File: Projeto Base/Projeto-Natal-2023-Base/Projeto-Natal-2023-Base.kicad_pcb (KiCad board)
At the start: 2 copper layers, 50 x 50 mm, 54 parts, among them J1 Conn_01x03_Pin, Q1 BC817, Q2 BC817, Q3 BC817, Q4 BC817, U1 CH32V003F4P6

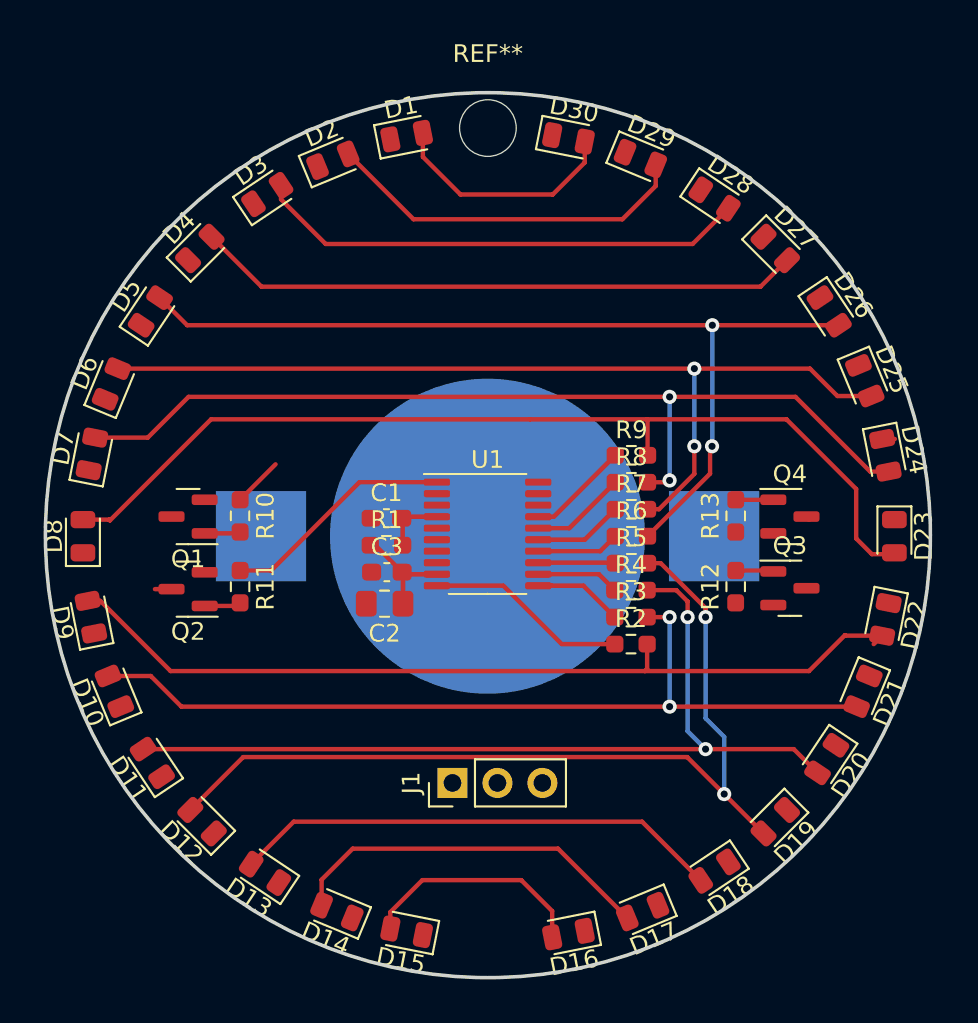
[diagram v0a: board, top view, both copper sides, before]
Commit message: v1.0.0
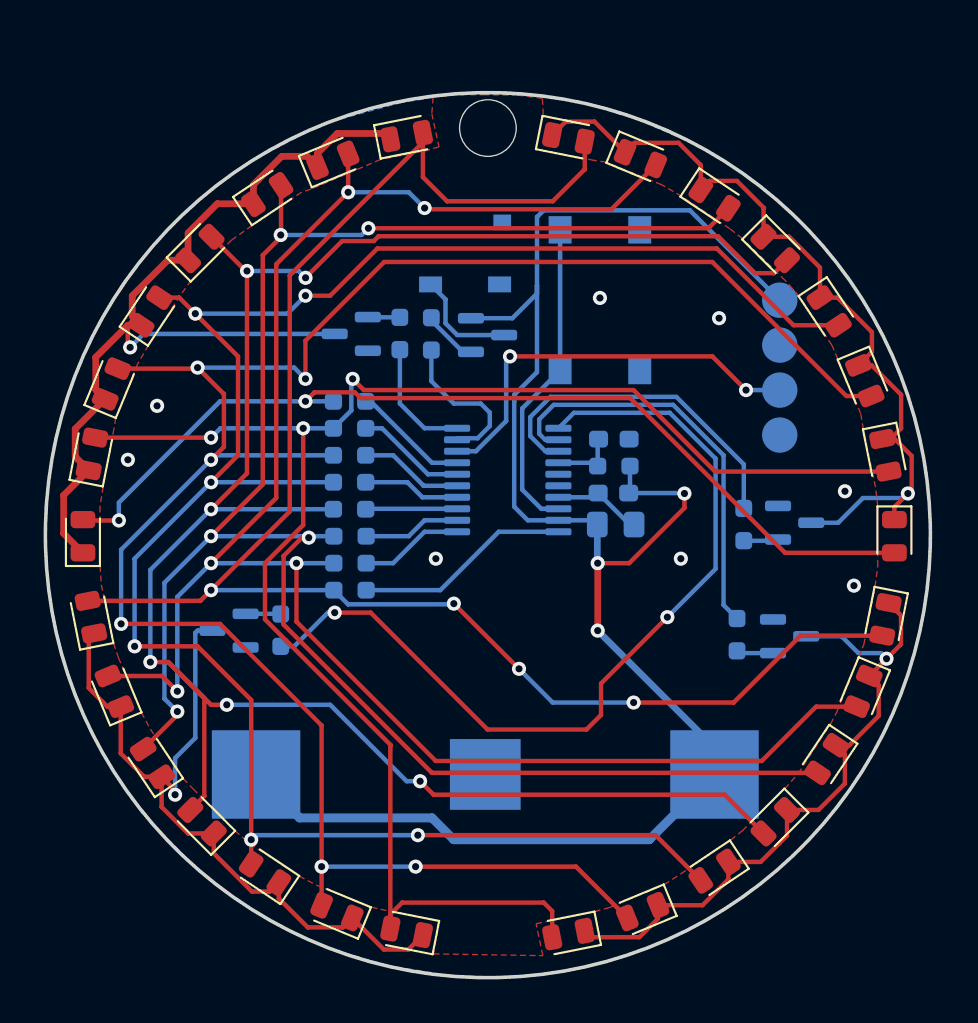
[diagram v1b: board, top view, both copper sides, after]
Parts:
- added BZ1: Buzzer, Library:PassiveBuzzerSMD_JiangsuHuaneng_MLT-5030, B.Cu at (92.7, 83.2)
- added J2: Conn_01x01_Pin, TestPoint:TestPoint_Pad_D2.0mm, B.Cu at (110.5, 85.7)
- added J3: Conn_01x01_Pin, TestPoint:TestPoint_Pad_D2.0mm, B.Cu at (110.5, 88.3)
- added J4: Conn_01x01_Pin, TestPoint:TestPoint_Pad_D2.0mm, B.Cu at (110.5, 90.8)
- added Q5: MMBT3906, Package_TO_SOT_SMD:SOT-23, B.Cu at (94.0, 87.7)
- added R14: 1K, Resistor_SMD:R_0603_1608Metric_Pad0.98x0.95mm_HandSolder, B.Cu at (90.8, 87.6)
- added SW1: SW_Push, Button_Switch_SMD:SW_Push_1P1T_NO_6x6mm_H9.5mm, B.Cu at (100.3, 85.7)
- BT1: footprint Battery:BatteryHolder_Keystone_3002_1x2032 -> Battery:BatteryHolder_Multicomp_BC-2001_1x2032
- C1, C2, C3, Q1, Q2, Q3, Q4, R1, R10, R11, R12, R13, R2, R3, R4, R5, R6, R7, R8, R9, U1: moved to B.Cu
- J1: value Conn_01x03_Pin -> Conn_01x01_Pin; footprint Connector_PinHeader_2.54mm:PinHeader_1x03_P2.54mm_Vertical -> TestPoint:TestPoint_Pad_D2.0mm; moved to B.Cu
- moved J1 27.0 mm to (110.5, 93.3), turned to -135 degrees
- moved R5 16.2 mm to (86.2, 97.5), turned to 180 degrees
- moved R6 16.2 mm to (86.2, 96.0), turned to 180 degrees
- moved R7 16.2 mm to (86.2, 94.5), turned to 180 degrees
- moved R8 16.2 mm to (86.2, 93.0), turned to 180 degrees
- moved R9 16.2 mm to (86.2, 91.4), turned to 180 degrees
- moved R2 16.2 mm to (86.2, 102.1), turned to 180 degrees
- moved R3 16.2 mm to (86.2, 100.6), turned to 180 degrees
- moved R4 16.2 mm to (86.2, 99.1), turned to 180 degrees
- moved Q1 13.8 mm to (86.3, 87.6)
- moved C2 13.8 mm to (101.2, 98.4), turned to 0 degrees
- moved R10 13.7 mm to (89.0, 87.6), turned to 90 degrees
- moved C1 13.6 mm to (101.1, 93.6), turned to 180 degrees
- moved R1 13.6 mm to (101.1, 95.1), turned to 180 degrees
- moved C3 13.6 mm to (101.1, 96.6)
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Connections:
- J1 pad 1: +3V3 -> unconnected-(J1-Pin_1-Pad1)
- U1 pad 19: unconnected-(U1-PD2-Pad19) -> BZR
- U1 pad 8: unconnected-(U1-PD0-Pad8) -> BT
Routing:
- net +3V3: track 6.63 -> 103.2 mm, vias 0 -> 3
- net Net-(D1-K): track 0.27 -> 54.6 mm, vias 0 -> 1
- net Net-(D23-K): track 0.98 -> 47.7 mm, vias 0 -> 1
- net Net-(D10-K): track 0.93 -> 45.1 mm, vias 0 -> 1
- net L6: track 73.7 -> 116.8 mm, vias 2 -> 6
- net Net-(D16-K): track 0.00 -> 38.5 mm, vias 0 -> 1
- net C2: track 13.2 -> 49.4 mm, vias 0 -> 2
- net L5: track 80.3 -> 114.9 mm, vias 2 -> 6
- net L2: track 70.2 -> 104.0 mm, vias 2 -> 5
- net L1: track 63.0 -> 94.8 mm, vias 0 -> 4
- net L4: track 85.0 -> 115.1 mm, vias 2 -> 6
- net L3: track 77.9 -> 107.9 mm, vias 2 -> 5
- net L7: track 66.6 -> 93.4 mm, vias 2 -> 3
- net C3: track 0.00 -> 23.5 mm
- net SWIO: track 0.00 -> 23.2 mm, vias 0 -> 2
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- added copper zone on B.Cu, net GND
- added copper zone on F.Cu, net GND
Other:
- board text added: "3V3"
- board text added: "GND"
- board text added: "NC"
- board text added: "SWIO"
